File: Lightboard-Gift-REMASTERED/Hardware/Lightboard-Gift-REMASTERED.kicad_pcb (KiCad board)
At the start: 2 copper layers, 90 x 62 mm, 30 parts, among them J1 USB_C_Receptacle_PowerOnly_6P, SW1 SW_Push, SW2 SW_SPST

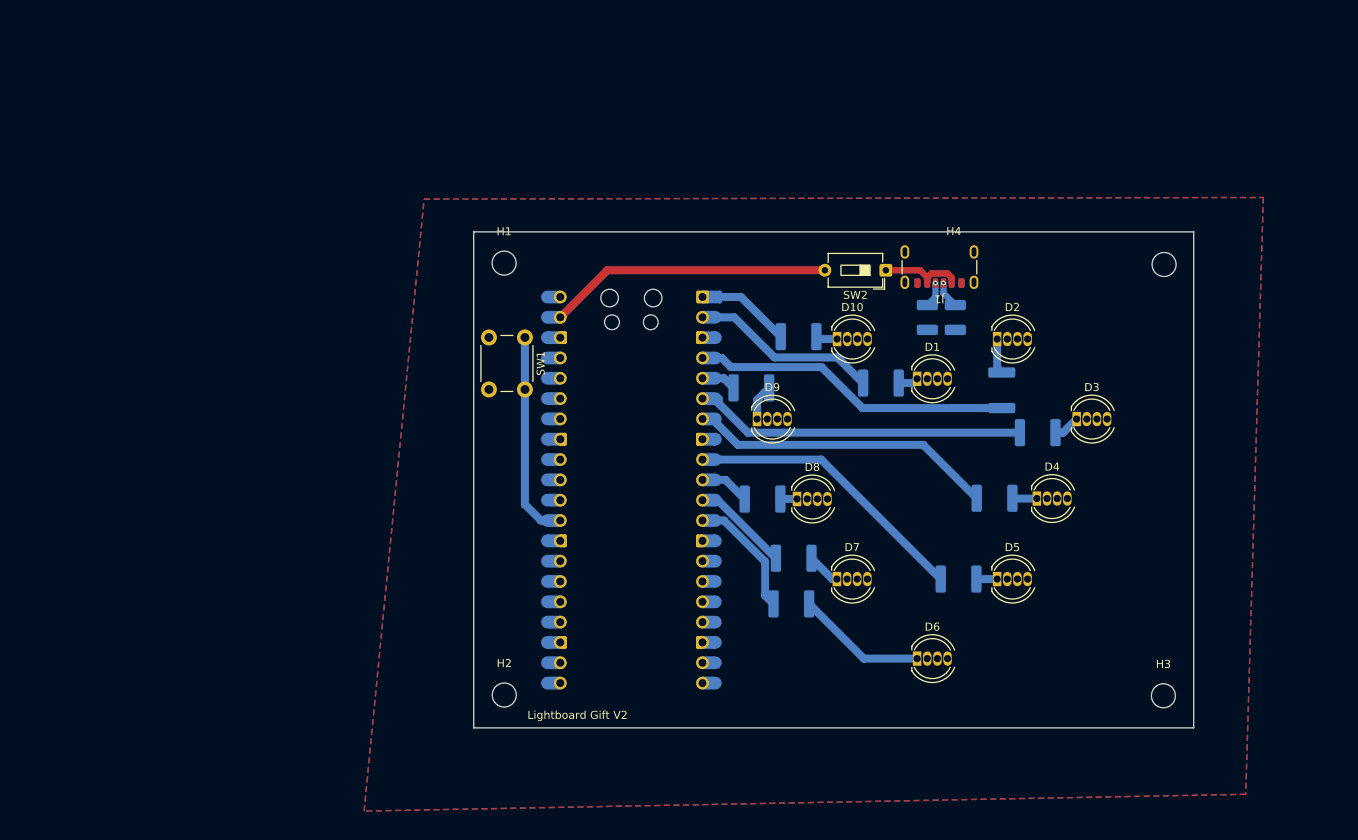
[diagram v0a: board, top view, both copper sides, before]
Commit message: V3 in the works!
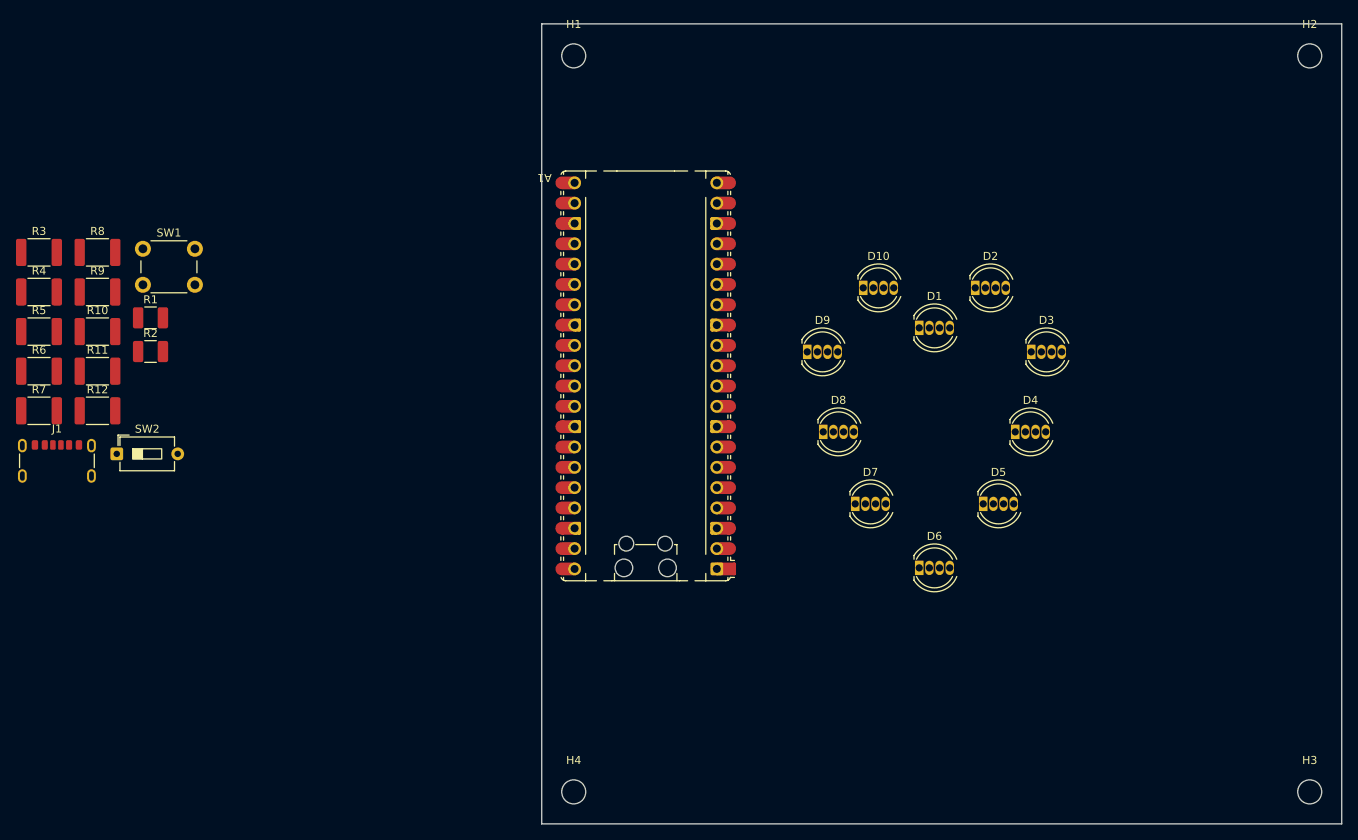
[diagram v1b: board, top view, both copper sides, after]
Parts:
- A1, R1, R10, R11, R12, R2, R3, R4, R5, R6, R7, R8, R9: moved to F.Cu
- moved H2 128.5 mm to (206.0, 34.0)
- moved R5 125.5 mm to (47.2, 68.5), turned to 0 degrees
- moved R4 121.0 mm to (47.2, 63.5), turned to 0 degrees
- moved R6 120.5 mm to (47.2, 73.4), turned to 0 degrees
- moved R7 116.8 mm to (47.2, 78.4), turned to 0 degrees
- moved J1 113.4 mm to (49.4, 85.7), turned to 0 degrees
- moved R3 106.5 mm to (47.2, 58.6), turned to 0 degrees
- moved R1 100.6 mm to (61.1, 66.7), turned to 0 degrees
- moved H4 99.0 mm to (114.0, 126.0)
- moved SW2 98.8 mm to (56.9, 83.8), turned to 0 degrees
- moved R8 97.2 mm to (54.5, 58.6), turned to 0 degrees
- moved R2 97.2 mm to (61.1, 71.0), turned to 0 degrees
- moved R9 93.2 mm to (54.5, 63.5), turned to 0 degrees
- moved R12 88.1 mm to (54.5, 78.4), turned to 0 degrees
- moved R10 85.7 mm to (54.5, 68.5), turned to 0 degrees
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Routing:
- net RED2: track 41.0 -> 0.00 mm
- net RED1: track 39.2 -> 0.00 mm
- net RED3: track 37.6 -> 0.00 mm
- net VBUS: track 35.5 -> 0.00 mm
- net RED4: track 35.2 -> 0.00 mm
- net Net-(A1-GPIO22): track 25.3 -> 0.00 mm
- net RED0: track 22.7 -> 0.00 mm
- net Net-(D6-RA): track 16.3 -> 0.00 mm
- net RED5: track 14.9 -> 0.00 mm
- net RED6: track 11.4 -> 0.00 mm
- net RED9: track 11.0 -> 0.00 mm
- net Net-(SW2-A): track 10.4 -> 0.00 mm
- net RED7: track 5.47 -> 0.00 mm
- net Net-(D9-RA): track 4.52 -> 0.00 mm
- net Net-(D2-RA): track 4.42 -> 0.00 mm
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- removed copper zone on B.Cu, net GND
- removed copper zone on F.Cu, net GND
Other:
- board size 90 x 62 mm -> 100 x 100 mm
- board text removed: "Lightboard Gift V2"
